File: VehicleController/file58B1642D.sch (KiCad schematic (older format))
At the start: 40 parts, among them J8 CONN_01X03, J9 CONN_02X12, Q4 Q_PMOS_GDS, Q5 PC_FET, Q6 PC_FET, U16 MC_Override, U17 MCR_Shtdwn, U18 MCL_Shtdwn, U19 RI-0505S, U20 ISO1540, U21 TCMT1103, U22 OPTO-TRANSISTOR-4, U23 PC_RLY, U24 MCP47FEBX2

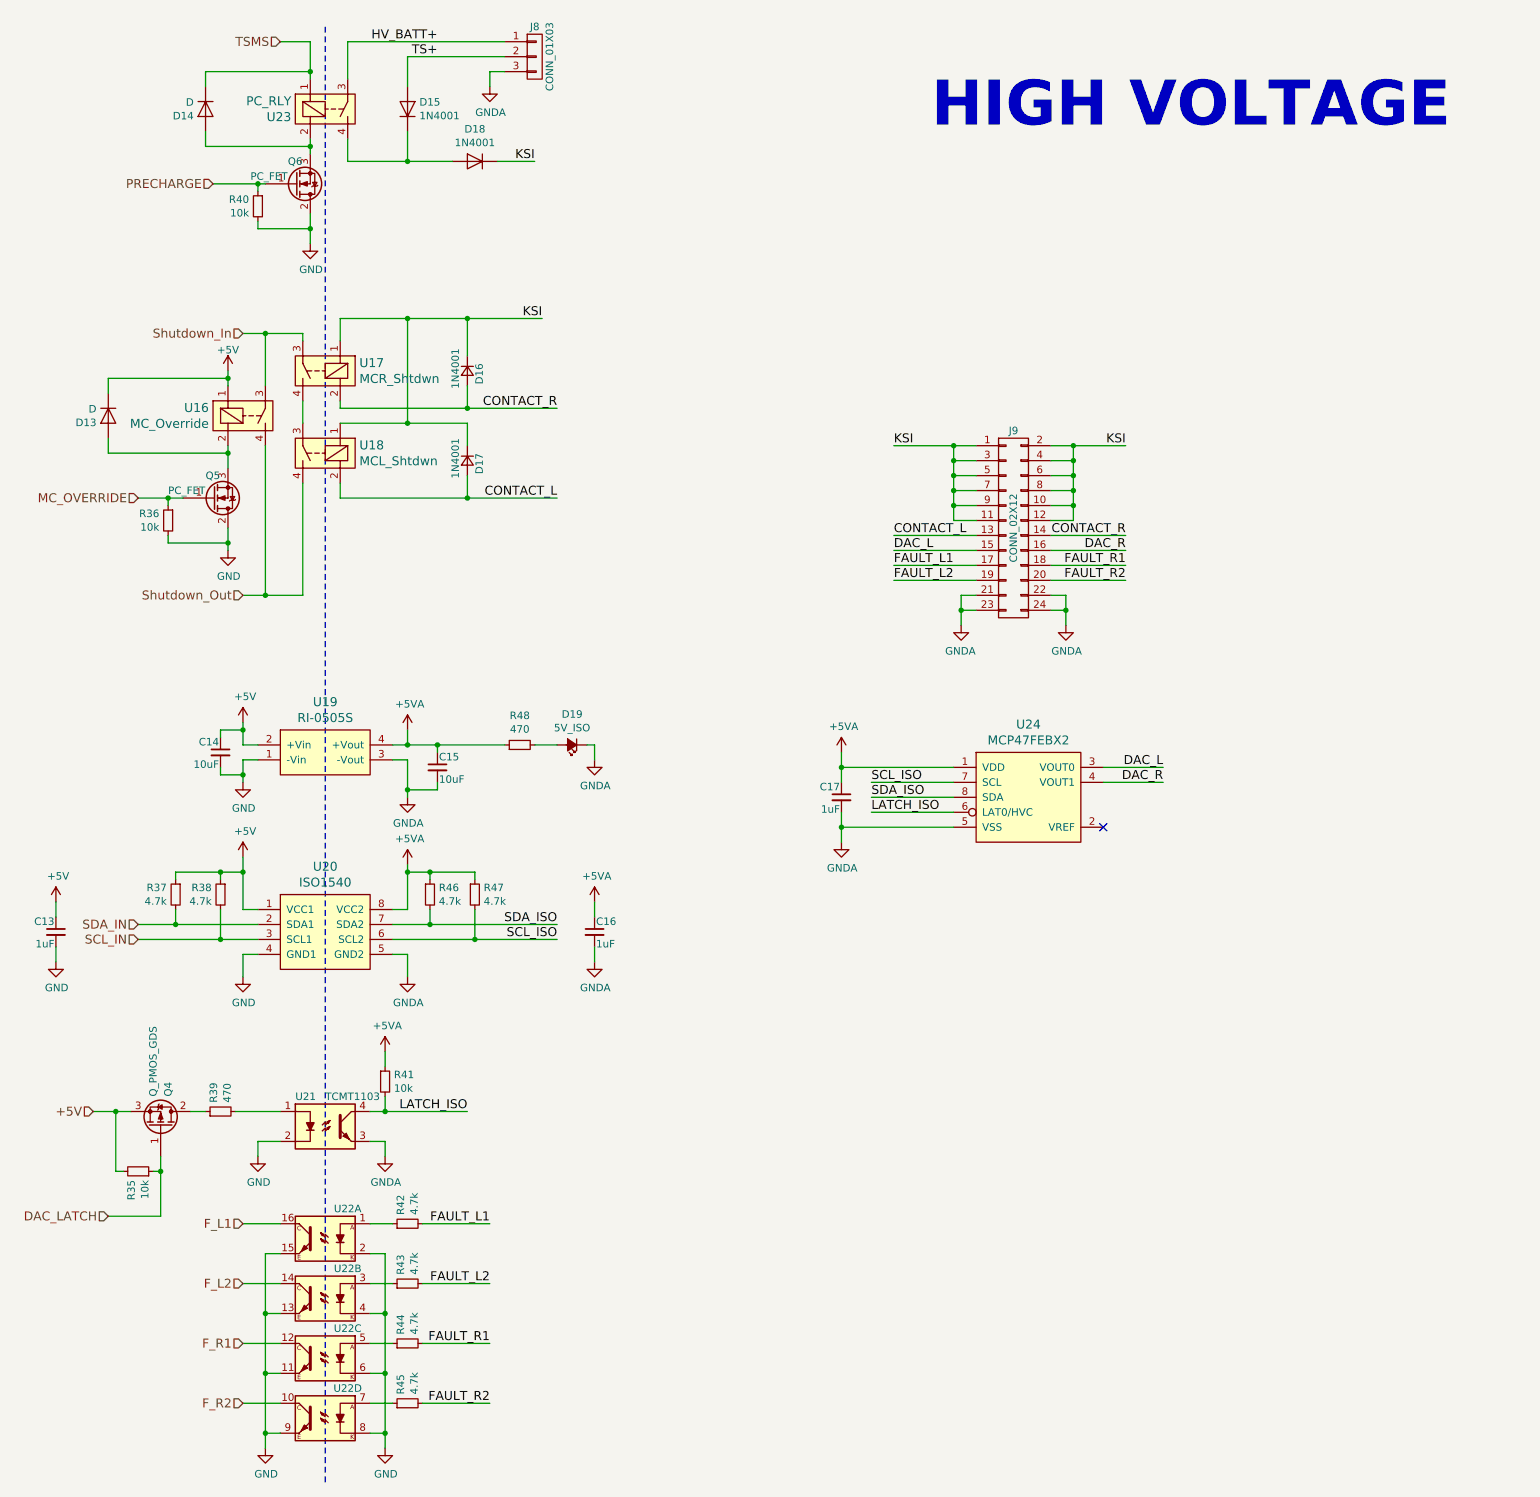
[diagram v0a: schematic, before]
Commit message: Small changes to VCU
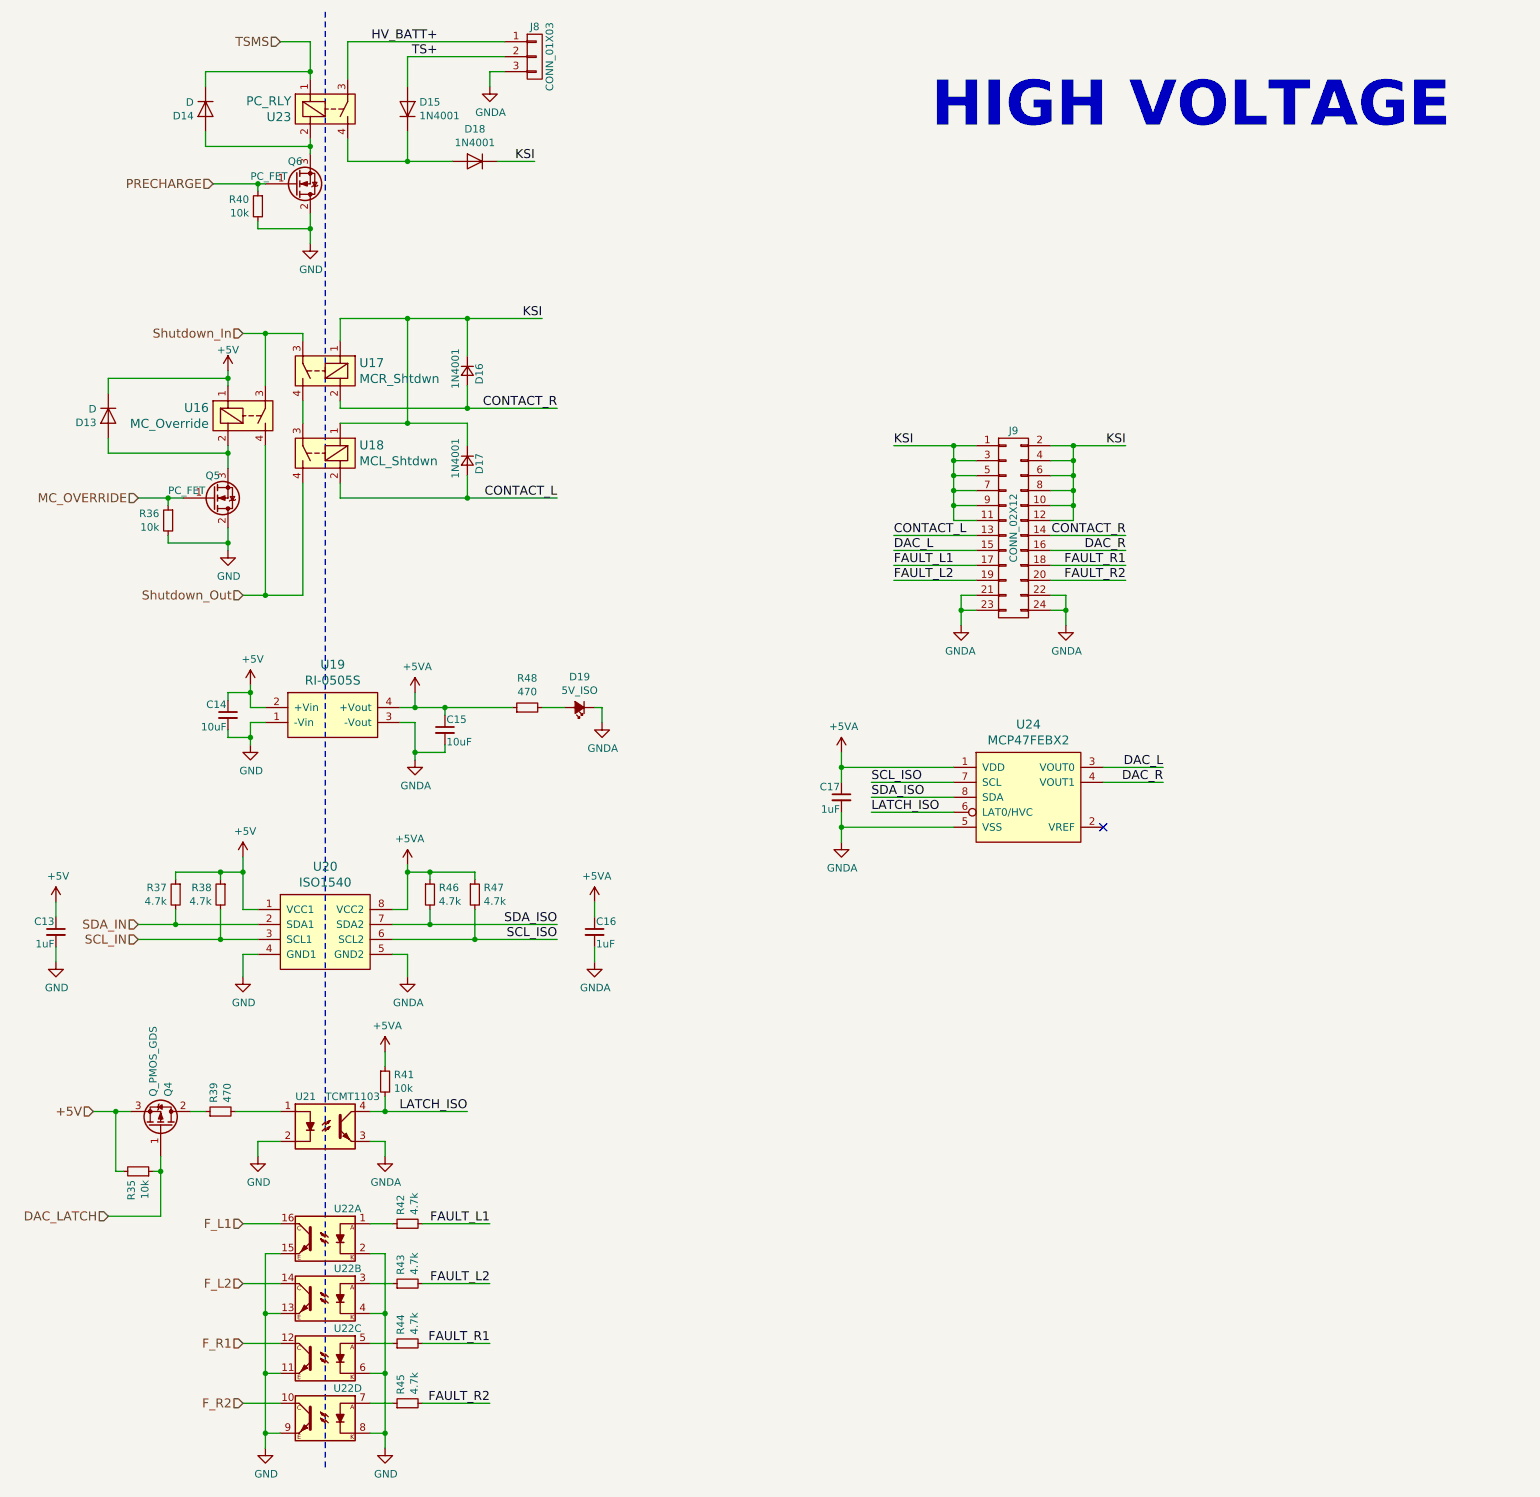
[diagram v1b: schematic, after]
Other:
- moved on the sheet: C14, C15, D19, R48, U19
